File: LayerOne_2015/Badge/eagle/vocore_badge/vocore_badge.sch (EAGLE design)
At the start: 17 parts

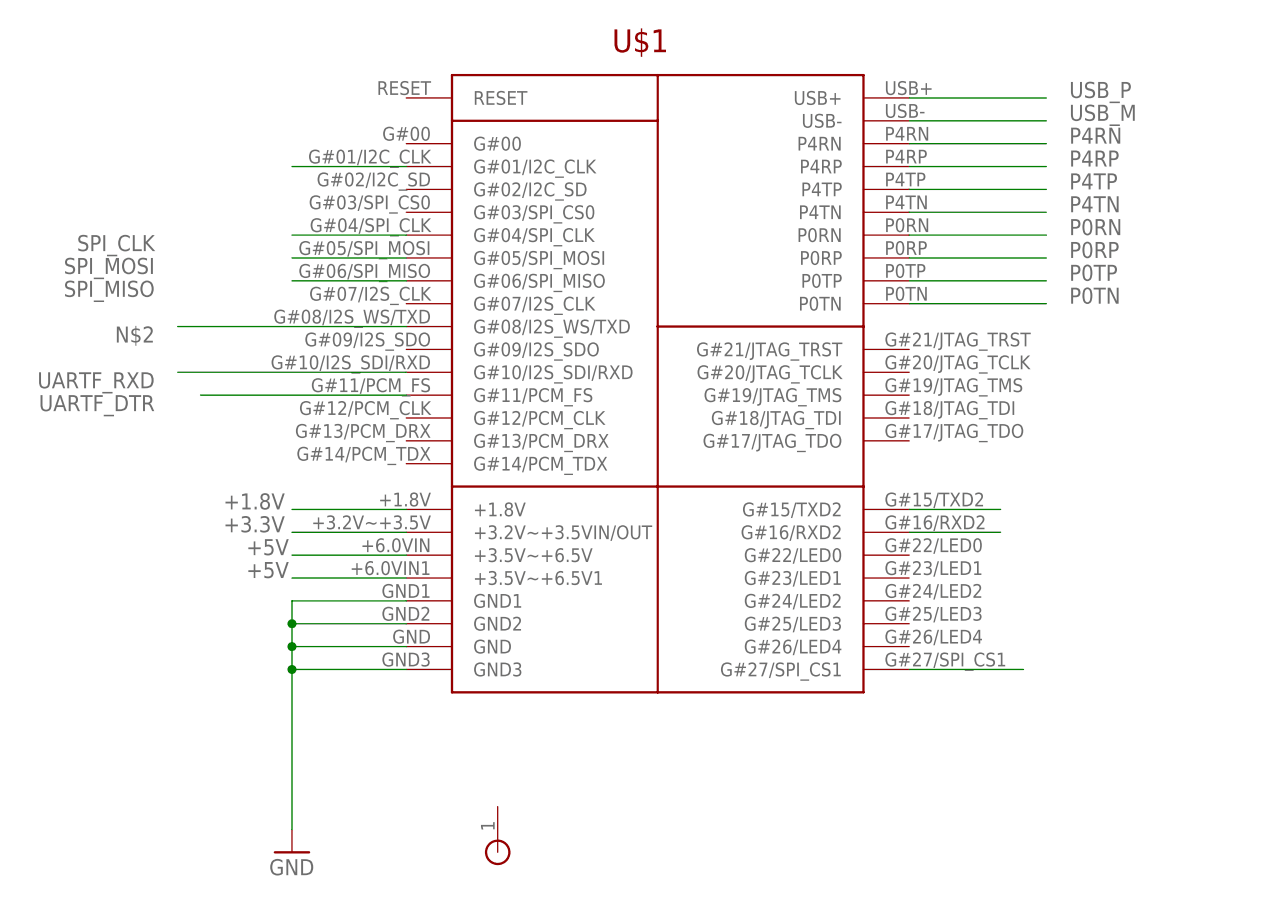
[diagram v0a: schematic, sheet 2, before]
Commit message: edited holes.
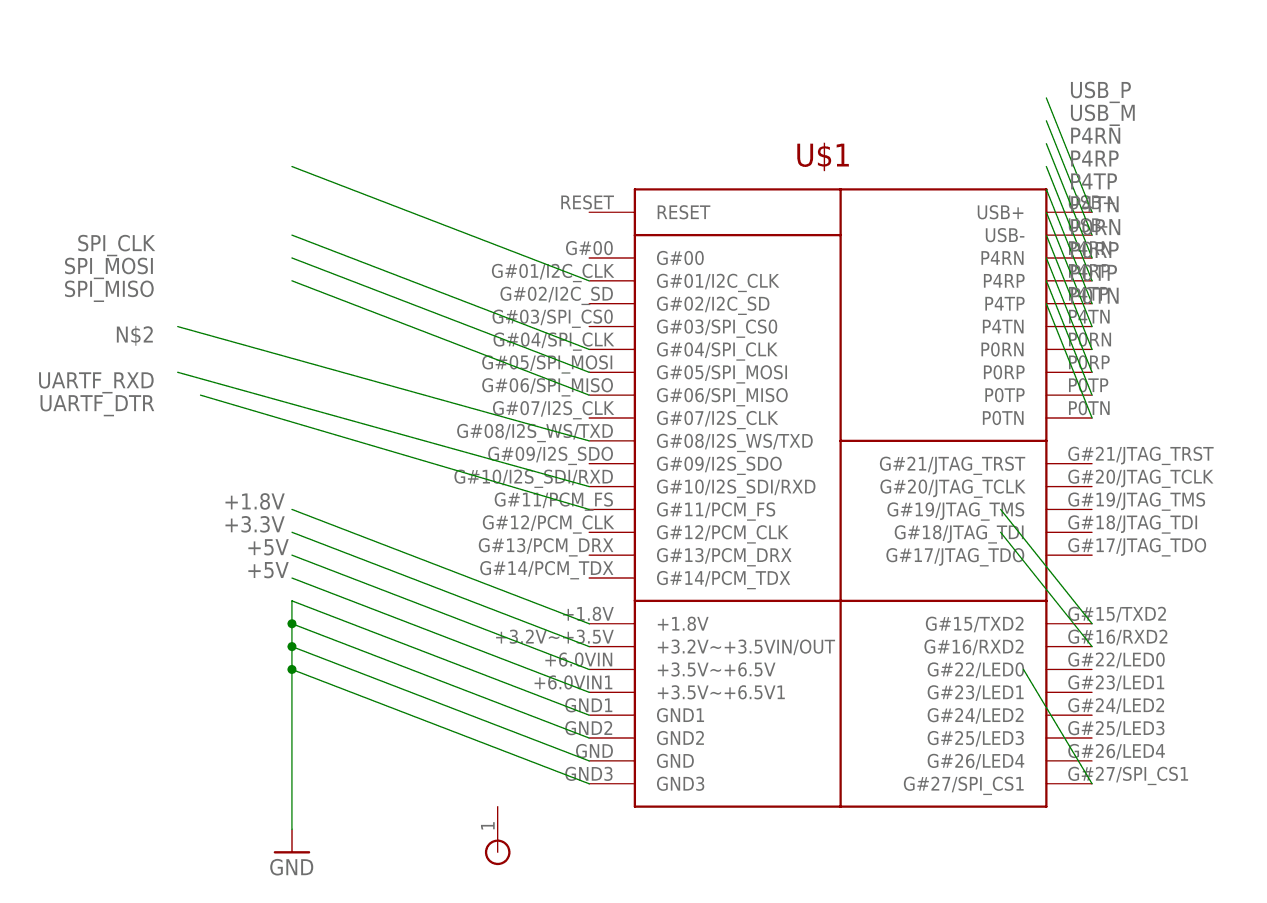
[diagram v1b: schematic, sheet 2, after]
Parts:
- R1, R10, R2, R3, R4, R5, R6, R7, R8, R9: value 0402_L -> (none); device vocore_dock:0402_L -> SparkFun-Resistors:RESISTOR0805-RES
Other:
- moved on the sheet: U$1
